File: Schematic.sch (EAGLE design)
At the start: 56 parts, among them IC1 74ALS09N, IC2 74AC04N, IC3 74AC08N, IC4 74AC04N, IC8 LM358N, Q1 IRF3205, Q2 IRF3205, Q3 IRF3205, Q4 IRF3205, X2 MOTOR DC, X3 Resistencia Shunt

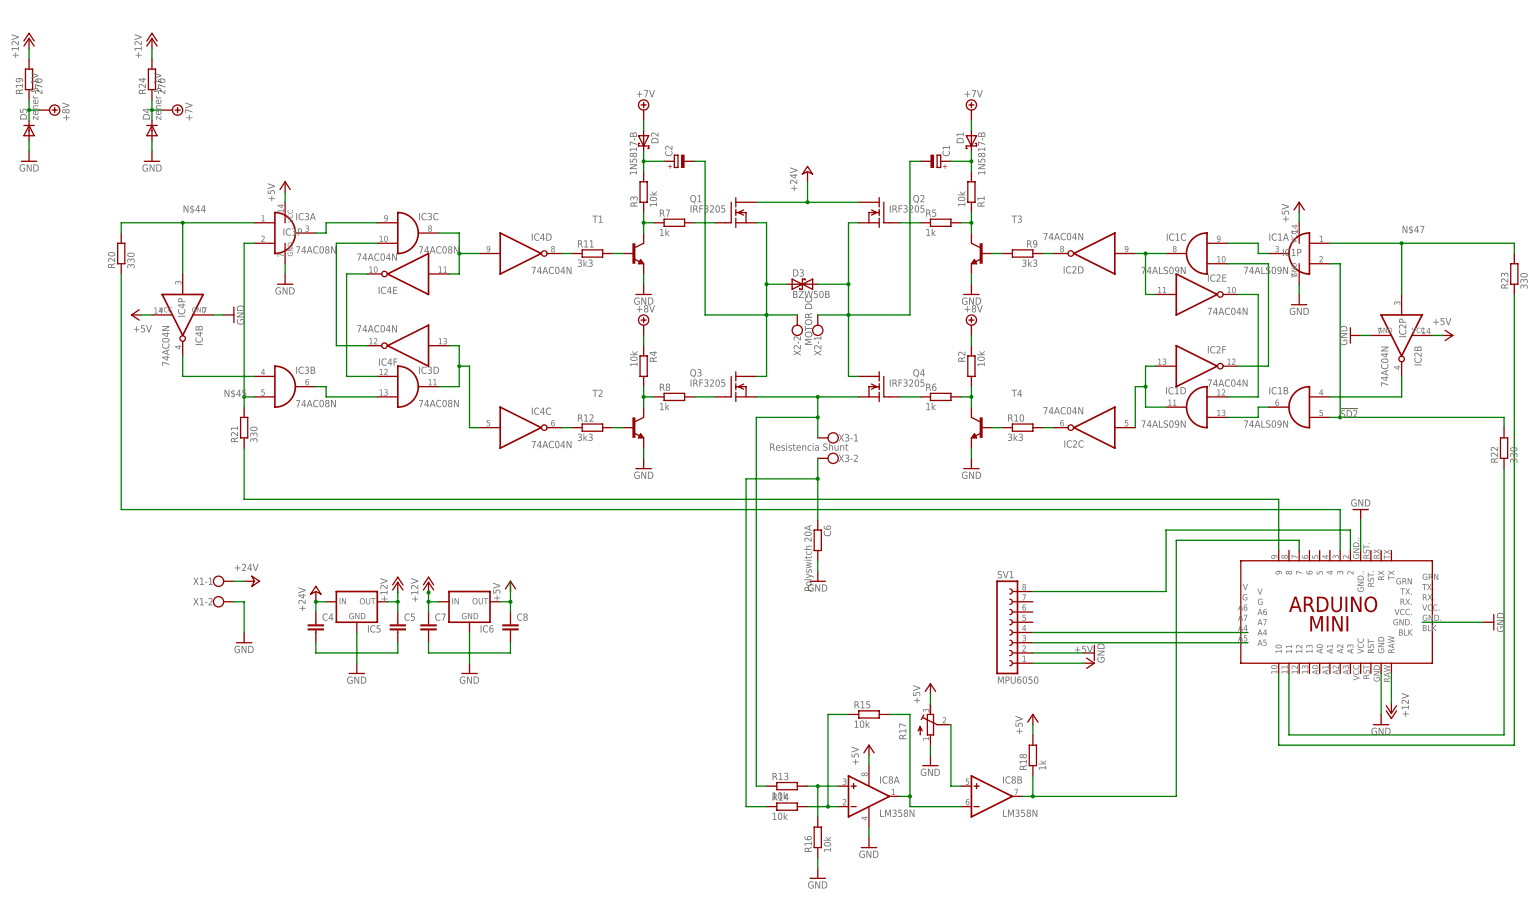
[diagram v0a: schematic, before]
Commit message: Ver 3
Board: Some adjustments at the design.
Algorithm:  Adjustments too.
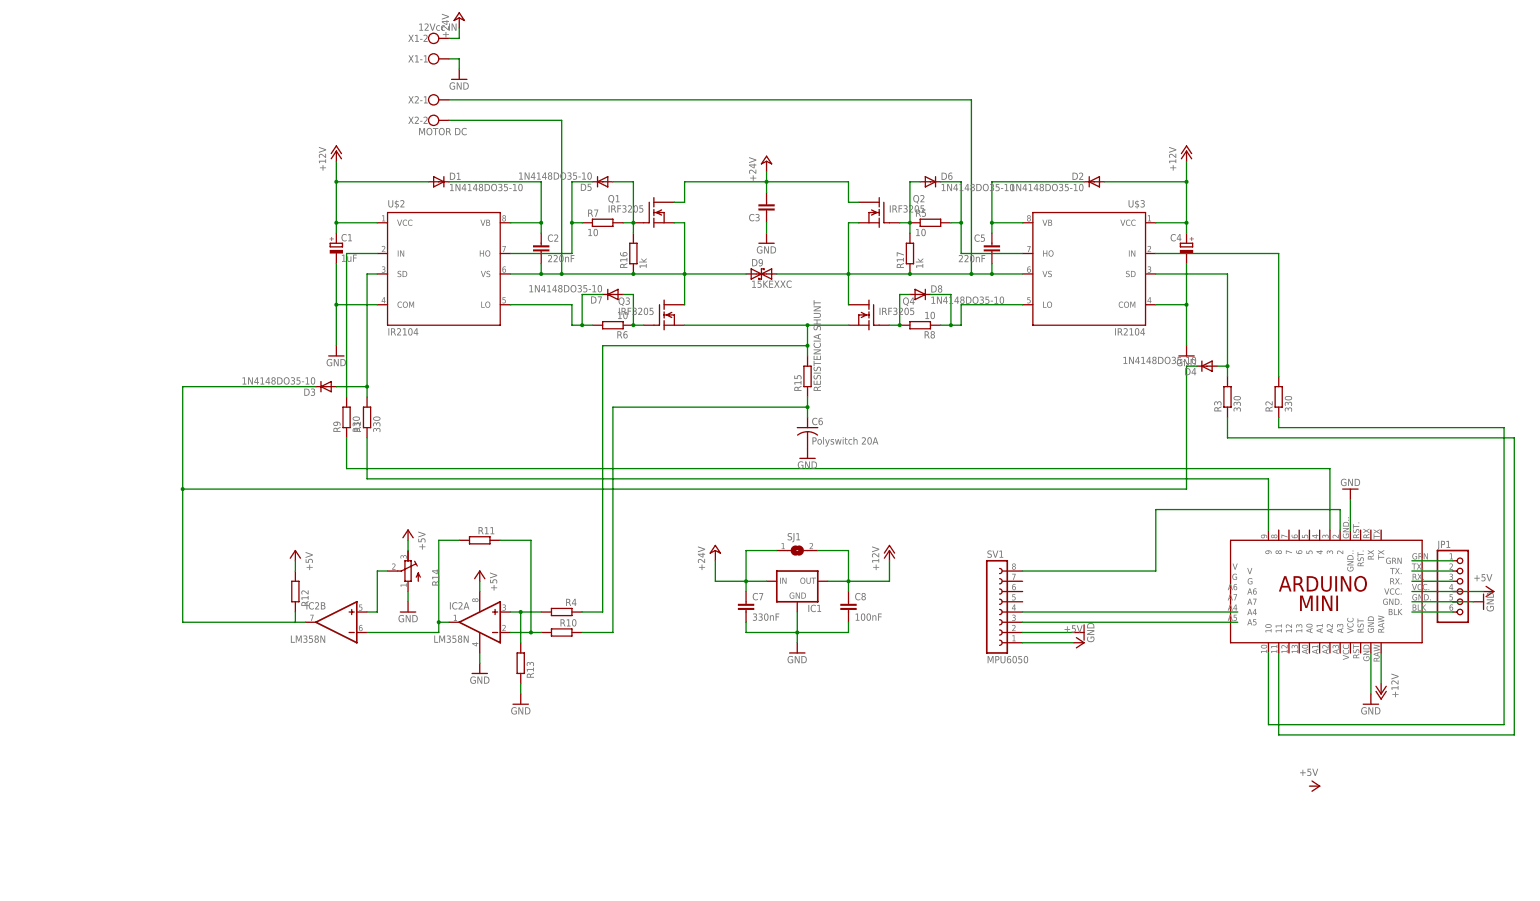
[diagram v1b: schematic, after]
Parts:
- removed IC3: 74AC08N, 74xx-eu:74AC08N
- removed IC4: 74AC04N, 74xx-eu:74AC04N
- removed IC5, IC6: (no value), v-reg:78XXL
- removed IC8: LM358N, linear:LM358N
- removed R18: 1k, rcl:R-EU_0204/7
- removed R19, R24: 270, rcl:R-EU_0207/12
- removed R20, R21, R22: 330, rcl:R-EU_0204/7
- removed R23: 330, rcl:R-EU_0207/10
- removed T1, T2, T3, T4: (no value), transistor:BC548-NPN-TO92-CBE
- removed X3: Resistencia Shunt, con-wago-500:W237-102
- added C3: (no value), rcl:C-EU050-030X075
- added D6, D7, D8: 1N4148DO35-10, diode:1N4148DO35-10
- added D9: 15KEXXC, diode:15KEXXC
- added JP1: (no value), pinhead:PINHD-1X6
- added SJ1: (no value), jumper:SJW
- added U$2, U$3: IR2104, IR2104:IR2104
- C1: value (none) -> 1uF; device rcl:CPOL-EUE3.5-10 -> rcl:CPOL-EUE3.5-8
- C2: value (none) -> 220nF; device rcl:CPOL-EUE3.5-10 -> rcl:C-EU075-032X103
- C4: device rcl:C-EU050-024X044 -> rcl:CPOL-EUE3.5-8
- C5: value (none) -> 220nF; device rcl:C-EU050-024X044 -> rcl:C-EU075-032X103
- C6: device rcl:R-EU_0309/12 -> rcl:C-US075-032X103
- C7: value (none) -> 330nF
- C8: value (none) -> 100nF
- D1, D2: value 1N5817-B -> 1N4148DO35-10; device diode:1N5817-B -> diode:1N4148DO35-10
- D3: value BZW50B -> 1N4148DO35-10; device diode:BZW50B -> diode:1N4148DO35-10
- D4, D5: value zener 5.1V -> 1N4148DO35-10; device diode:BYX90G -> diode:1N4148DO35-10
- IC1: value 74ALS09N -> (none); device 74xx-eu:74ALS09N -> v-reg:78XXL
- IC2: value 74AC04N -> LM358N; device 74xx-eu:74AC04N -> linear:LM358N
- Q1, Q2, Q3, Q4: device transistor-fet:BUZ50A -> transistor-fet Victor:BUZ10
- R1, R2, R3: value 10k -> 330
- R10: value 3k3 -> (none); device rcl:R-EU_0207/12 -> rcl_Victor:R-EU_0204/7
- R11, R12: value 3k3 -> (none); device rcl:R-EU_0204/7 -> rcl_Victor:R-EU_0204/7
- R13, R4: value 10k -> (none); device rcl:R-EU_0204/7 -> rcl_Victor:R-EU_0204/7
- R14: value 10k -> (none); device rcl:R-EU_0204/7 -> rcl_Victor:R-TRIMM64W
- R15: value 10k -> RESISTENCIA SHUNT; device rcl:R-EU_0204/7 -> resistor:R-EU_0922V
- R16: value 10k -> 1k; device rcl:R-EU_0204/7 -> rcl:R-EU_0207/10
- R17: value (none) -> 1k; device rcl:R-TRIMM64W -> rcl:R-EU_0207/10
- R5: value 1k -> 10; device rcl:R-EU_0204/7 -> rcl:R-EU_0207/12
- R6, R7: value 1k -> 10; device rcl:R-EU_0204/7 -> rcl:R-EU_0207/10
- R8: value 1k -> 10; device rcl:R-EU_0204/7 -> rcl:R-EU_0207/15
- R9: value 3k3 -> 330; device rcl:R-EU_0207/15 -> rcl:R-EU_0207/10
- X1: value (none) -> 12Vcc IN
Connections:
- removed net !SD1: R21.1, U$1.9
- removed net !SD2: IC1A.I1, IC1B.I1, R22.2
- removed net +7V: D1.A, D2.A, D4.C, D5.C, R19.1, R2.1, R24.1, R4.1
- removed net IN1: R20.1, U$1.3
- removed net IN2: R23.1, U$1.10
- removed net N$12: R9.2, T3.B
- removed net N$14: IC1D.I0, IC2E.O
- removed net N$17: IC1C.I1, IC2F.O
- removed net N$29: IC3D.I0, IC4E.O
- removed net N$30: IC3C.I1, IC4F.O
- removed net N$35: IC8A.-IN, R14.2, R15.1
- removed net N$36: R3.1, R7.1, T1.C
- removed net N$38: IC8A.OUT, IC8B.-IN, R15.2
- removed net N$39: R11.2, T1.B
- removed net N$40: IC8B.OUT, R18.1, U$1.7
- removed net N$41: R12.2, T2.B
- removed net N$43: C6.1, R14.1, X3-2.KL
- removed net N$44: IC3A.I0, IC4B.I, R20.2
- removed net N$45: IC3A.I1, IC3B.I1, R21.2
- removed net N$47: IC1A.I0, IC2B.I, R23.2
- removed net N$49: R22.1, U$1.11
- removed net N$53: IC2C.O, R10.2
- removed net N$54: IC2D.O, R9.1
- removed net N$55: IC4D.O, R11.1
- removed net N$56: IC1D.O, IC2C.I, IC2F.I
- new net N$22: IC2A.OUT, IC2B.-IN, R11.2
- new net N$48: JP1.6, U$1.BLK
- new net N$5: R2.2, U$3.IN
- new net N$50: JP1.3, U$1.RX.
- new net N$51: JP1.2, U$1.TX.
- new net N$52: JP1.1, U$1.GRN
- net +12V: now also C1.+, C4.+, C8.1, D1.A, D2.A, IC1.OUT, SJ1.2, U$2.VCC, U$3.VCC; no longer C5.1, C7.1, IC5.OUT, IC6.IN, R19.2, R24.2
- net +24V: now also C3.2, C7.1, IC1.IN, SJ1.1, X1-2.KL; no longer C4.1, IC5.IN, X1-1.KL
- net +5V: now also IC2P.V+, JP1.4, R12.2, R14.E, U$1.VCC.; no longer C8.1, IC1P.VCC, IC2P.VCC, IC3P.VCC, IC4P.VCC, IC6.OUT, IC8P.V+, R17.E, R18.2
- net GND: now also C1.-, C3.1, C4.-, IC1.GND, IC2P.V-, JP1.5, R13.1, R14.A, U$2.COM, U$3.COM, X1-1.KL; no longer C4.2, C5.2, D4.A, D5.A, IC1P.GND, IC2P.GND, IC3P.GND, IC4P.GND, IC5.GND, IC6.GND, IC8P.V-, R16.1, R17.A, T1.E, T2.E, T3.E, T4.E, X1-2.KL
- net N$1: now also R9.2, U$2.IN; no longer C1.+, D1.C, R1.2
- net N$10: now also R9.1, U$1.3; no longer IC4C.O, R12.1
- net N$11: now also D8.A, Q4.G; no longer Q3.G
- net N$13: now also C2.2, D9.1, R16.1, U$2.VS; no longer C2.-, D3.1
- net N$16: now also C5.2, D9.2, R17.1, U$3.VS; no longer C1.-, D3.2
- net N$18: now also R15.2, R4.1; no longer R13.1, X3-1.KL
- net N$19: now also R2.1, U$1.10; no longer IC1B.O, IC1D.I1
- net N$2: now also C2.1, D1.C, U$2.VB; no longer C2.+, D2.C, R3.2
- net N$20: now also C5.1, D2.C, U$3.VB; no longer IC1A.O, IC1C.I0
- net N$23: now also D5.C, R7.1, U$2.HO; no longer IC1B.I0, IC2B.O
- net N$24: now also D7.C, R6.2, U$2.LO; no longer IC8B.+IN, R17.S
- net N$25: now also D8.C, R8.1, U$3.LO; no longer R2.2, R6.2, T4.C
- net N$26: now also D6.C, R5.2, U$3.HO; no longer R10.1, T4.B
- net N$27: now also IC2A.+IN, R13.2; no longer R8.1, T2.C
- net N$28: now also D3.A, R1.2, U$2.SD; no longer IC3D.O, IC4C.I, IC4F.I
- net N$3: now also D5.A, R16.2
- net N$31: now also IC2A.-IN, R10.2, R11.1; no longer IC3A.O, IC3C.I0
- net N$32: now also IC2B.+IN, R14.S; no longer IC3B.O, IC3D.I1
- net N$33: now also R3.1, U$1.11; no longer IC8A.+IN, R13.2, R16.2
- net N$34: now also C6.1, R10.1, R15.1; no longer IC3B.I0, IC4B.O
- net N$4: now also D6.A, R17.2
- net N$6: now also D4.A, R3.2, U$3.SD; no longer IC3C.O, IC4D.I, IC4E.I
- net N$7: now also U$1.9; no longer R5.2, T3.C
- net N$8: now also D3.C, D4.C, IC2B.OUT, R12.1; no longer IC1C.O, IC2D.I, IC2E.I
- net N$9: now also D7.A, Q3.G; no longer Q4.G
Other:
- note removed: "NOTAS IMPORTANTES: *Los transistores de la base de los fets tienen q ser tipo BC548.. Puede q mas adelante haya q reemplazarlos por fets chiquitos. *Hay q regular bien la tension de los transistores de gate para q qde limitado en corriente. *Chequear pero parece q las AND estas son OPEN-COLLECTOR.. Hay q cambiarlas por las comunes q son 08. *Hay q agregar la entrada del medidor de corriente al ar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"
- moved on the sheet: C1, C5, C6, C7, C8, Q1, Q3, Q4, R1, R10, R11, R12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
